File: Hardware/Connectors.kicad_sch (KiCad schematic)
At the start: 41 parts, among them J10 USB_C_Receptacle, J13 JST_Locking_6, J14 Qwiic_Vertical, J2 SMA_Edge, J3 Conn_01x15, J4 Conn_01x18, J5 JST_Locking_6, J6 SMA_Edge, J7 USB_C_Receptacle, J8 U.FL, J9 U.FL

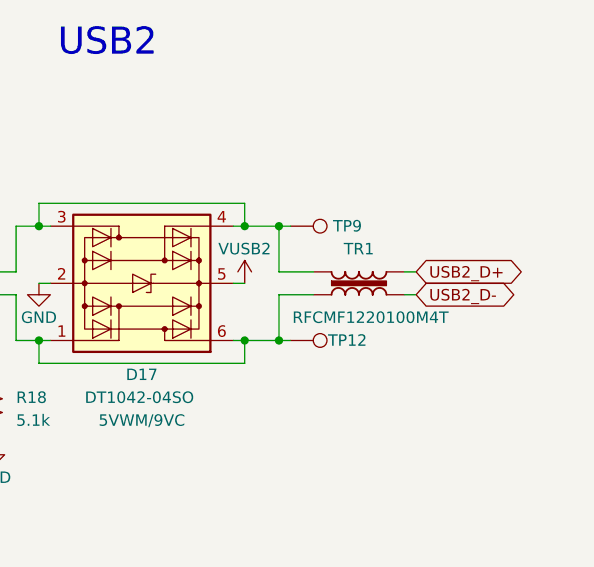
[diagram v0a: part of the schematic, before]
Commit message: Routing WIP
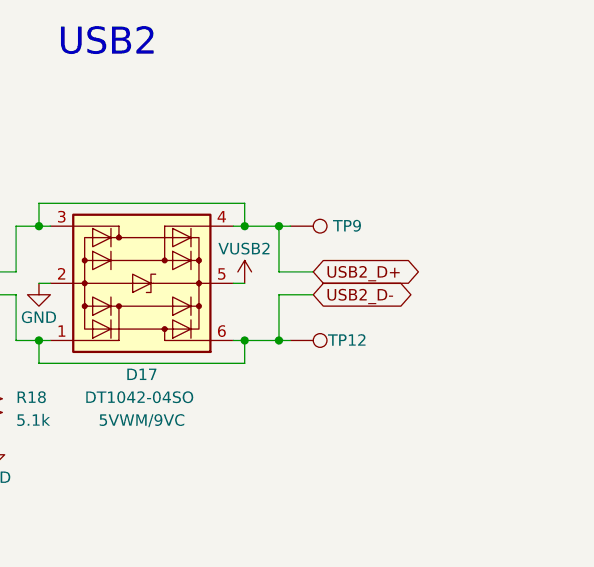
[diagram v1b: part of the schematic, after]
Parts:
- removed TR1: RFCMF1220100M4T, SparkFun-Coil:RFCMF1220100M4T, symbol SparkFun-Coil:USB_Transformer
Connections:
- net USB2_D+: now also D17.3 (I/O2), D17.4 (I/O3), J7.A6 (D+), J7.B6 (D+), TP9.1
- net USB2_D-: now also D17.1 (I/O1), D17.6 (I/O4), J7.A7 (D-), J7.B7 (D-), TP12.1
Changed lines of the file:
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@@
 	(wire
 		(pts
-			(xy 247.65 115.57) (xy 248.92 115.57)
-		)
-		(stroke
-			(width 0)
-			(type default)
-		)
-	)
-	(wire
-		(pts
 			(xy 142.24 52.07) (xy 142.24 60.96)
 		)
@@
 	(wire
 		(pts
-			(xy 247.65 113.03) (xy 248.92 113.03)
-		)
-		(stroke
-			(width 0)
-			(type default)
-		)
-	)
-	(wire
-		(pts
 			(xy 195.58 33.02) (xy 195.58 34.29)
 		)
@@
 	(global_label "USB2_D-"
 		(shape bidirectional)
-		(at 248.92 115.57 0)
+		(at 237.49 115.57 0)
 		(fields_autoplaced yes)
 		(effects
@@
 		)
 		(property "Intersheetrefs" "${INTERSHEET_REFS}"
-			(at 261.846 115.57 0)
+			(at 250.416 115.57 0)
 			(effects
 				(font
@@
 	(global_label "USB2_D+"
 		(shape bidirectional)
-		(at 248.92 113.03 0)
+		(at 237.49 113.03 0)
 		(fields_autoplaced yes)
 		(effects
@@
 		)
 		(property "Intersheetrefs" "${INTERSHEET_REFS}"
-			(at 261.846 113.03 0)
+			(at 250.416 113.03 0)
 			(effects
 				(font
@@
 					(unit 1)
 				)
-			)
-		)
-	)
-	(symbol
-		(lib_id "SparkFun-Coil:USB_Transformer")
-		(at 242.57 114.3 0)
-		(mirror x)
-		(unit 1)
-		(exclude_from_sim no)
-		(in_bom yes)
-		(on_board yes)
-		(dnp no)
-		(property "Reference" "TR1"
-			(at 242.57 110.49 0)
-			(effects
-				(font
-					(size 1.27 1.27)
-				)
-			)
-		)
-		(property "Value" "RFCMF1220100M4T"
-			(at 243.84 118.11 0)
-			(effects
-				(font
-					(size 1.27 1.27)
-				)
-			)
-		)
-		(property "Footprint" "SparkFun-Coil:RFCMF1220100M4T"
-			(at 241.3 107.95 0)
-			(effects
-				(font
-					(size 1.27 1.27)
-				)
-				(hide yes)
-			)
-		)
-		(property "Datasheet" "http://www.passivecomponent.com/wp-content/uploads/2018/10/RF-Filter.pdf"
-			(at 241.3 105.41 0)
-			(effects
-				(font
-					(size 1.27 1.27)
-				)
-				(hide yes)
-			)
-		)
-		(property "Description" "USB Transformer"
-			(at 242.57 100.33 0)
-			(effects
-				(font
-					(size 1.27 1.27)
-				)
-				(hide yes)
-			)
-		)
-		(property "PROD_ID" "COMP-19495"
-			(at 241.3 102.87 0)
-			(effects
-				(font
-					(size 1.27 1.27)
-				)
-				(hide yes)
-			)
-		)
-		(pin "1"
-		)
-		(pin "2"
-		)
-		(pin "4"
-		)
-		(pin "3"
-		)
-		(instances
-			(project ""
-				(path "/e3dd3ae4-244d-4cba-9cca-5d2abf83f29a/31a2c60b-91be-4113-ae16-f797035e304d"
-					(reference "TR1")
-					(unit 1)
-				)
